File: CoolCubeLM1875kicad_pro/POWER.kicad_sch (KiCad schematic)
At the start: 47 parts, among them IC7 TPS7A4901, J1 AC, J2 AC, J3 GND, J5 GND, J6 GND, J9 GND, K2 STBY RELAY, U3 LMR51430, U7 TPS7A39

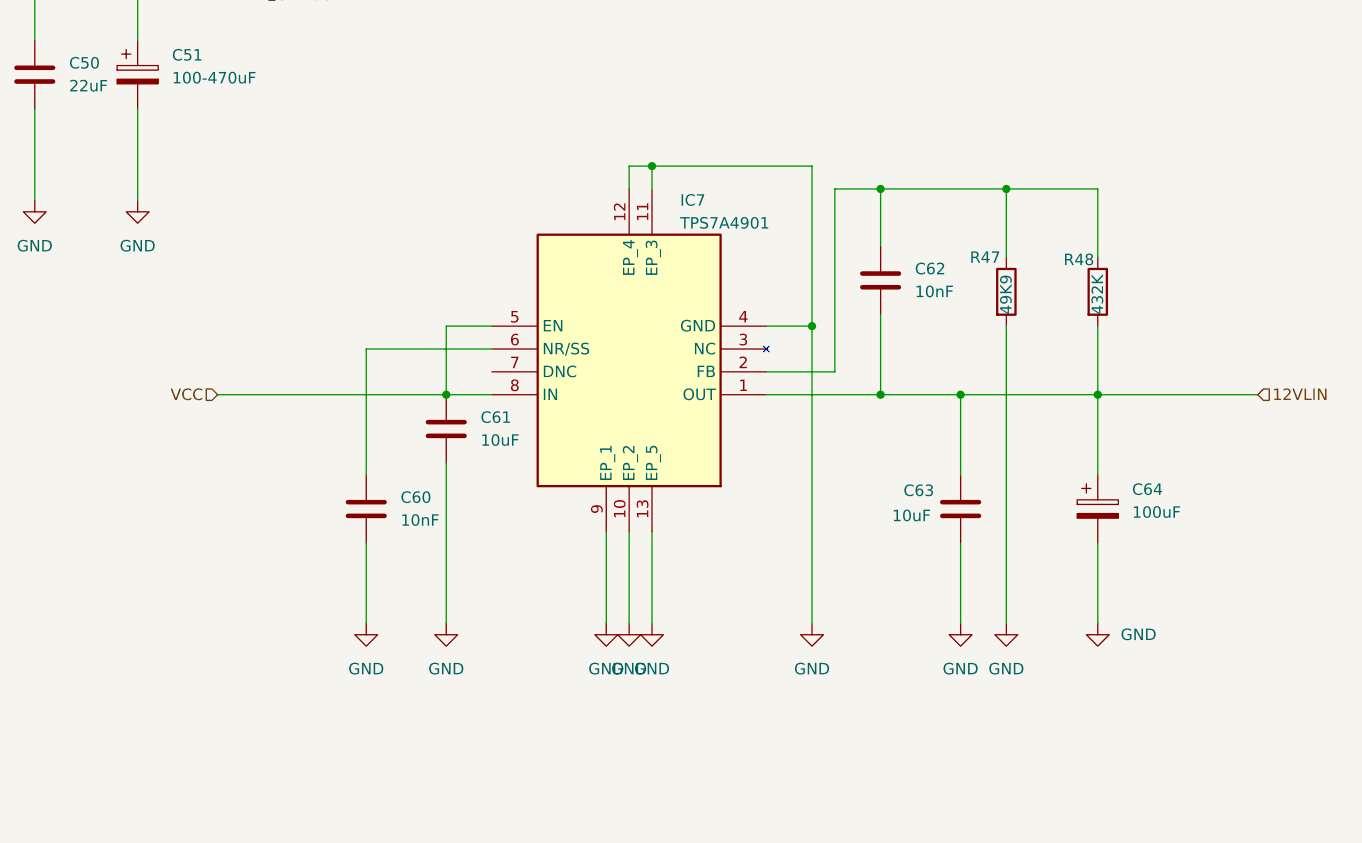
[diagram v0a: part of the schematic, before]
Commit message: final design
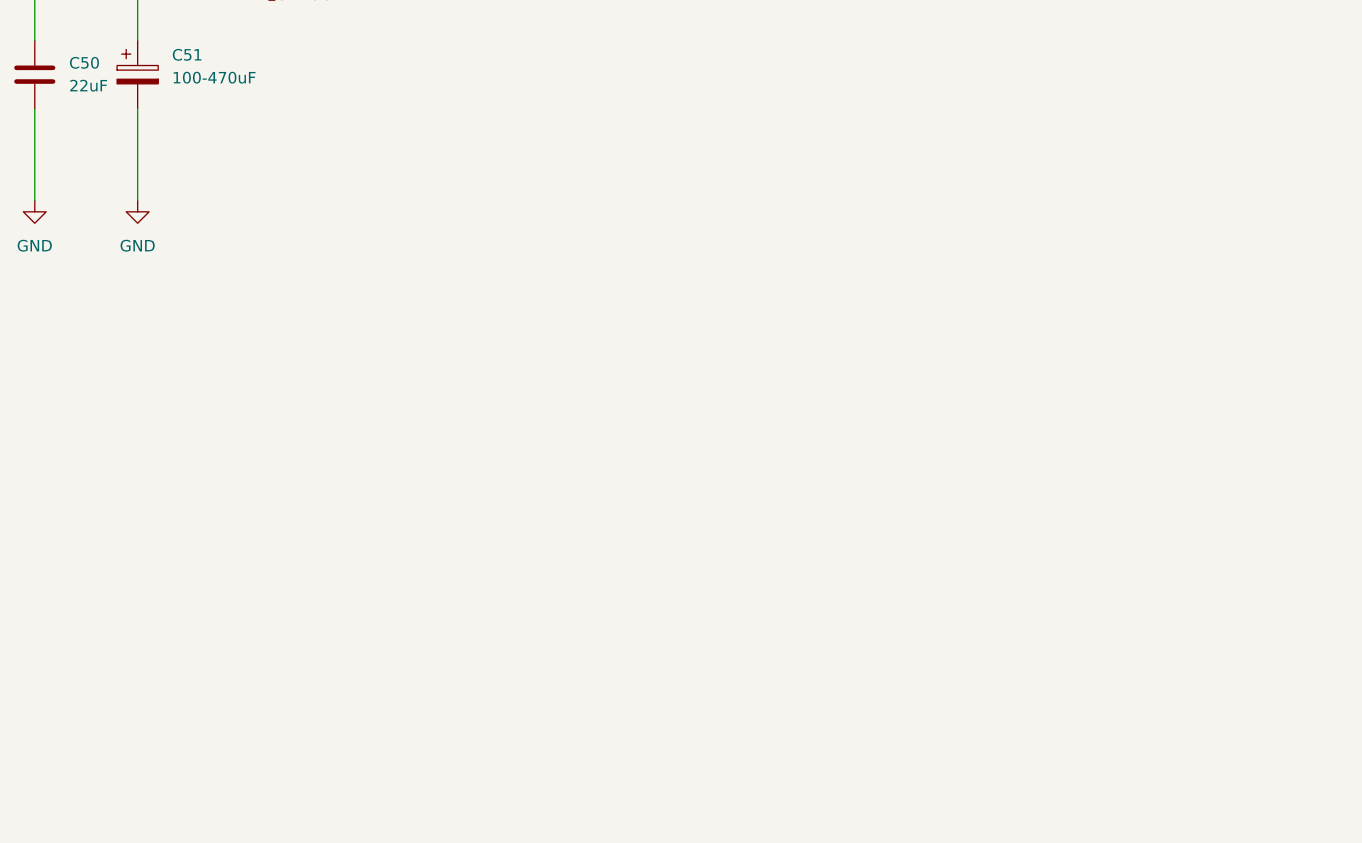
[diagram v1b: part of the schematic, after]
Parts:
- removed C60, C62: 10nF, Capacitor_SMD:C_0805_2012Metric_Pad1.18x1.45mm_HandSolder, symbol Device:C
- removed C61, C63: 10uF, Capacitor_SMD:C_1206_3216Metric_Pad1.33x1.80mm_HandSolder, symbol Device:C
- removed C64: 100uF, Capacitor_THT:CP_Radial_D6.3mm_P2.50mm, symbol Device:C_Polarized
- removed IC7: TPS7A4901, Custom:TPS7A4901DRBR, symbol Custom:TPS7A4901DRBR
- removed R47: 49K9, Resistor_SMD:R_0805_2012Metric_Pad1.20x1.40mm_HandSolder, symbol Device:R
- removed R48: 432K, Resistor_SMD:R_0805_2012Metric_Pad1.20x1.40mm_HandSolder, symbol Device:R

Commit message: more
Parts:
- J1, J2, J3, J5, J6, J9: footprint Spade connector:TE_62409-1 -> (none)
